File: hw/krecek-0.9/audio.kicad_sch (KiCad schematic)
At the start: 8 parts, among them CN1 PJ-313B6-B, U10 TPA2028D1YZFT, U11 ES8312

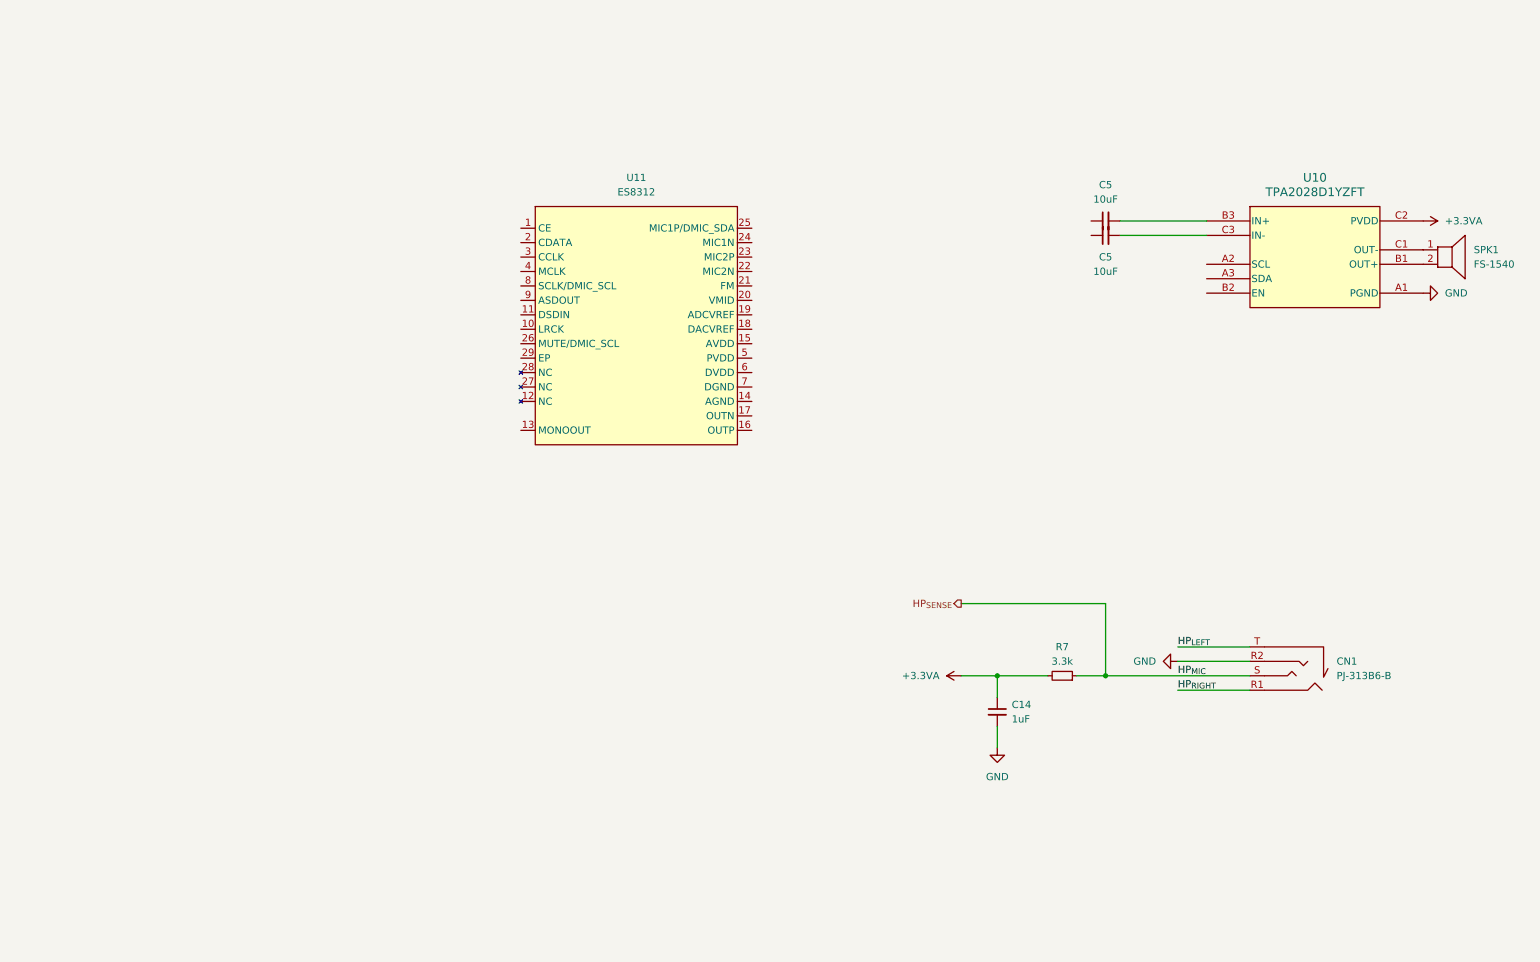
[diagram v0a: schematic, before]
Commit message: Complete most of the design, except for RF
Signed-off-by: Jan Hamal Dvořák <mordae@anilinux.org>
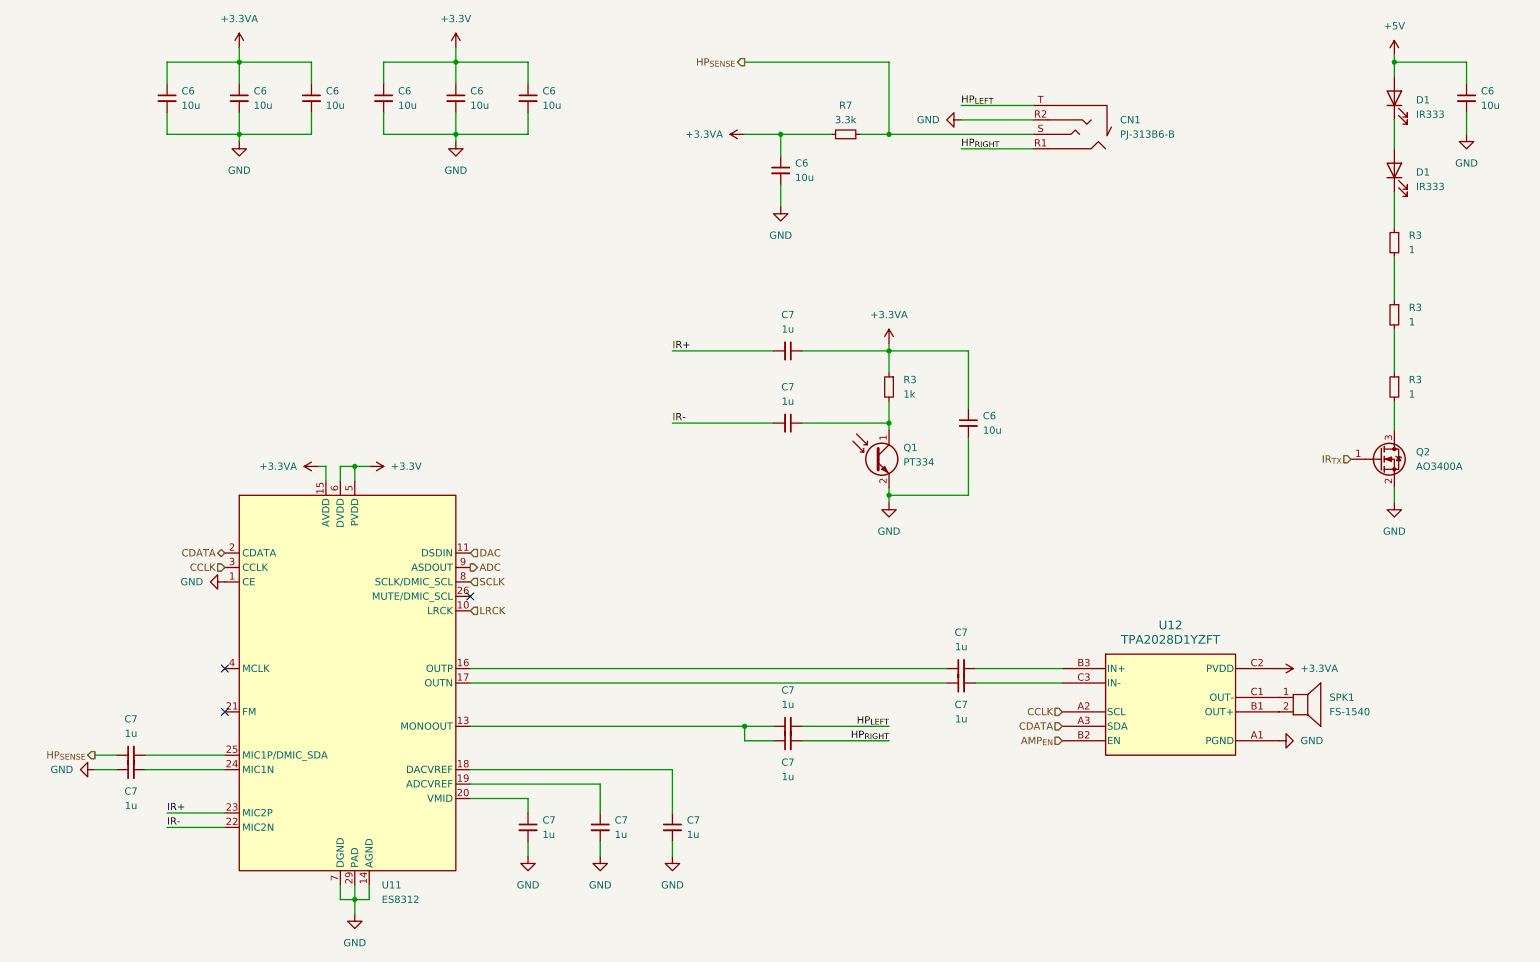
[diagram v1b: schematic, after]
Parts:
- removed C14: 1uF, Capacitor_SMD:C_0805_2012Metric, symbol Device:C_Small
- removed C5 (x2): 10uF, Capacitor_SMD:C_0805_2012Metric, symbol Device:C_Small
- added C6 (x9): 10u, Capacitor_SMD:C_0402_1005Metric, symbol Device:C_Small
- added C7 (x11): 1u, Capacitor_SMD:C_0402_1005Metric, symbol Device:C_Small
- added D1 (x2): IR333, LED_THT:LED_D5.0mm_Horizontal_O1.27mm_Z3.0mm_Clear, symbol Device:LED
- added Q1: PT334, LED_THT:LED_D5.0mm_Horizontal_O1.27mm_Z3.0mm_IRBlack, symbol Device:Q_Photo_NPN
- added Q2: AO3400A, Package_TO_SOT_SMD:SOT-23, symbol Transistor_FET:AO3400A
- added R3 (x3): 1, Resistor_SMD:R_1206_3216Metric, symbol Device:R_Small
- added R3: 1k, Resistor_SMD:R_0402_1005Metric, symbol Device:R_Small
- renumbered U10 to U12
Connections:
- net +3.3VA: now also U11.15 (AVDD), C6.1, C6.1, C6.1, C6.1, C6.1, C7.1, R3.1
- net GND: now also U11.1 (CE), U11.14 (AGND), U11.29 (PAD), U11.7 (DGND), C6.2, C6.2, C6.2, C6.2, C6.2, C6.2, C6.2, C6.2, C6.2, C7.1, C7.2, C7.2, C7.2, Q1.2 (E), Q2.2 (S)
- net HP_{LEFT}: now also C7.2
- net HP_{RIGHT}: now also C7.2
- net HP_{SENSE}: now also C7.1
- net LRCK: now reaches U11.10 (LRCK)
- net DAC: now reaches U11.11 (DSDIN)
- net at U11.13 (MONOOUT): now also C7.1, C7.1
- net at U11.16 (OUTP): now also C7.1
- net at U11.17 (OUTN): now also C7.1
- net at U11.18 (DACVREF): now also C7.1
- net at U11.19 (ADCVREF): now also C7.1
- net CDATA: now reaches U11.2 (CDATA)
- net CDATA: now also U12.A3 (SDA)
- net at U11.20 (VMID): now also C7.1
- net IR-: now reaches U11.22 (MIC2N)
- net IR-: now also C7.2
- net IR+: now reaches U11.23 (MIC2P)
- net IR+: now also C7.2
- net at U11.24 (MIC1N): now also C7.2
- net at U11.25 (MIC1P/DMIC_SDA): now also C7.2
- net CCLK: now reaches U11.3 (CCLK)
- net CCLK: now also U12.A2 (SCL)
- net +3.3V: now reaches U11.5 (PVDD)
- net +3.3V: now also U11.6 (DVDD), C6.1, C6.1, C6.1
- net SCLK: now reaches U11.8 (SCLK/DMIC_SCL)
- net ADC: now reaches U11.9 (ASDOUT)
- net at SPK1.3: no longer SPK1.4
- net AMP_{EN}: now reaches U12.B2 (EN)
- net at U12.B3 (IN+): now also C7.2
- net at U12.C3 (IN-): now also C7.2
- new net: Q2.3 (D), R3.2
- new net: C7.1, Q1.1 (C), R3.2
- new net: R3.1, R3.2 (x2)
- new net: D1.1 (K), R3.1
- new net: D1.1 (K), D1.2 (A)
- new net +5V: C6.1, D1.2 (A)
- new net IR_{TX}: Q2.1 (G)
- no-connect marks 0 -> 3
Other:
- moved on the sheet: CN1, R7, SPK1, U12
